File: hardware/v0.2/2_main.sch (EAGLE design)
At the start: 80 parts, among them IC1 SN74LVC1G08, IC2 FP6291, J1 RJ9PTH, Q1 PMOS, Q2 8050, Q3 MOSFET-NCHANNELBSS138, Q4 MOSFET-NCHANNELBSS138, U1 STM32F10XRXT6, Y1 8M

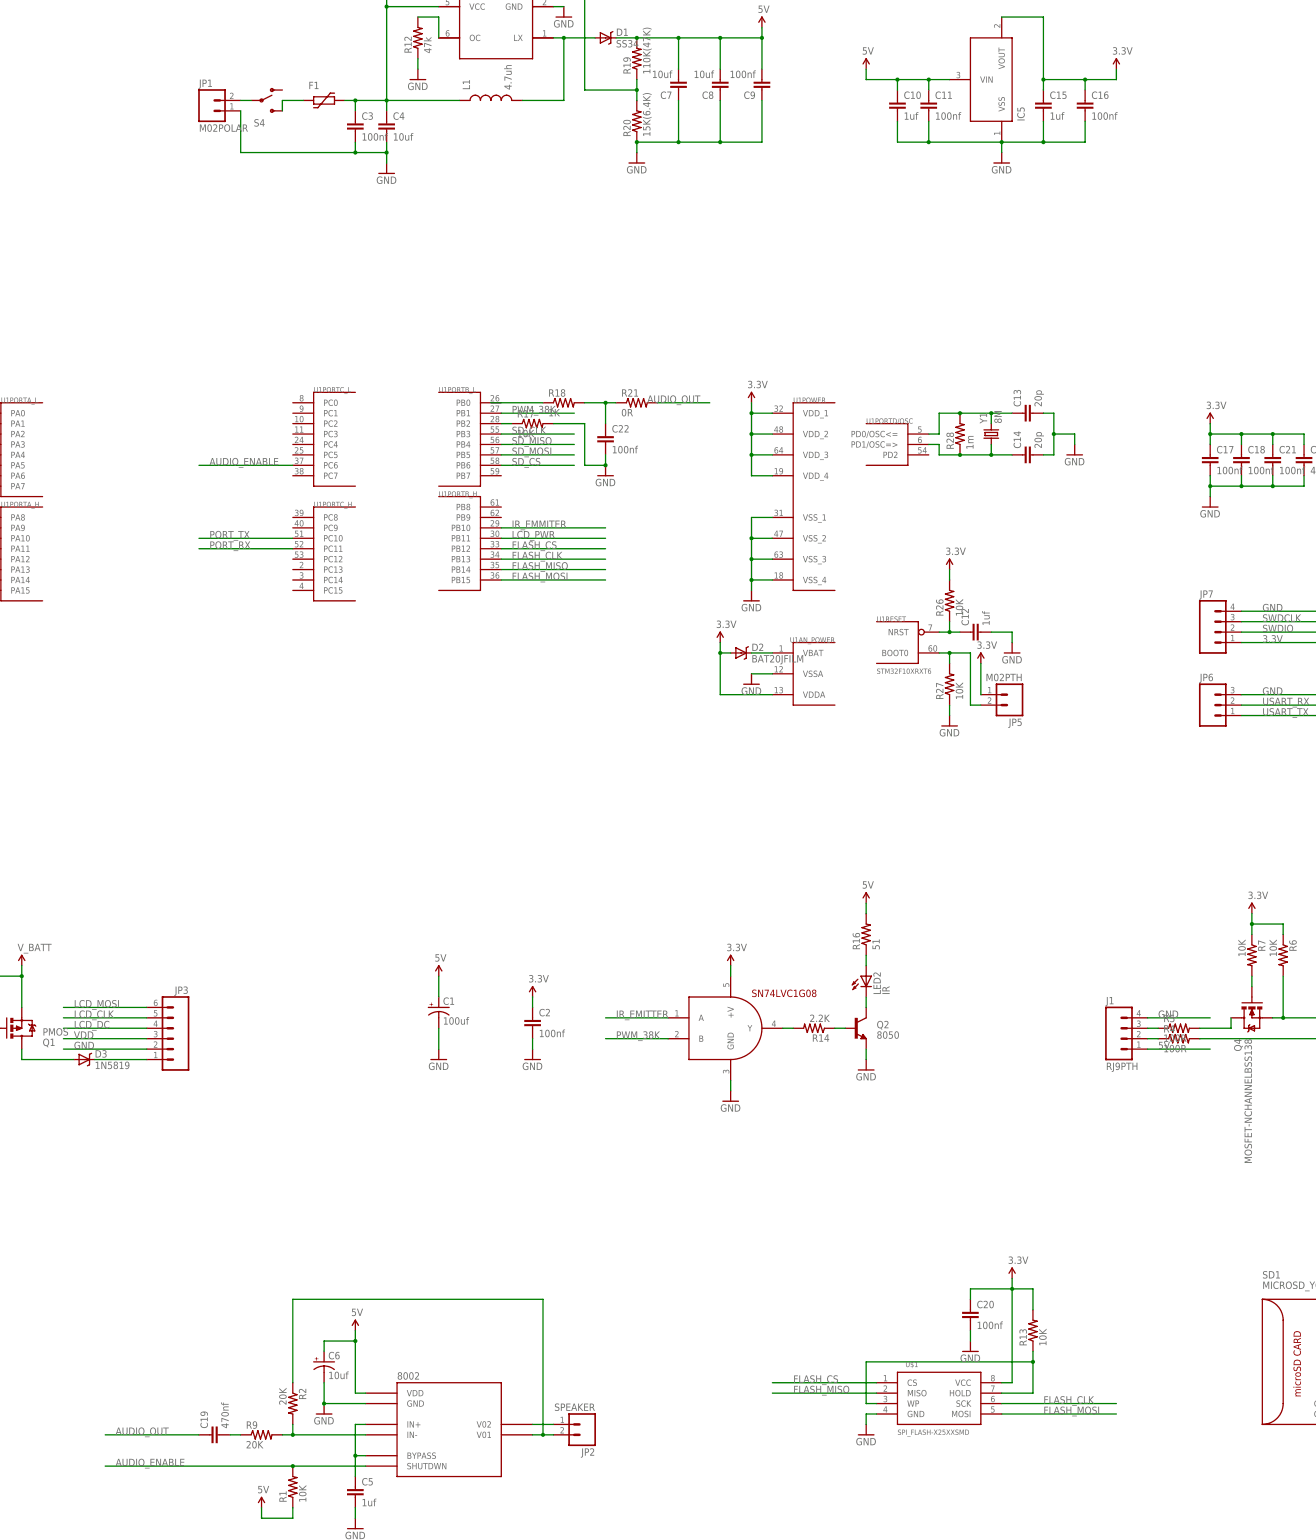
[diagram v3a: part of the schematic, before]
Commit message: update pcb
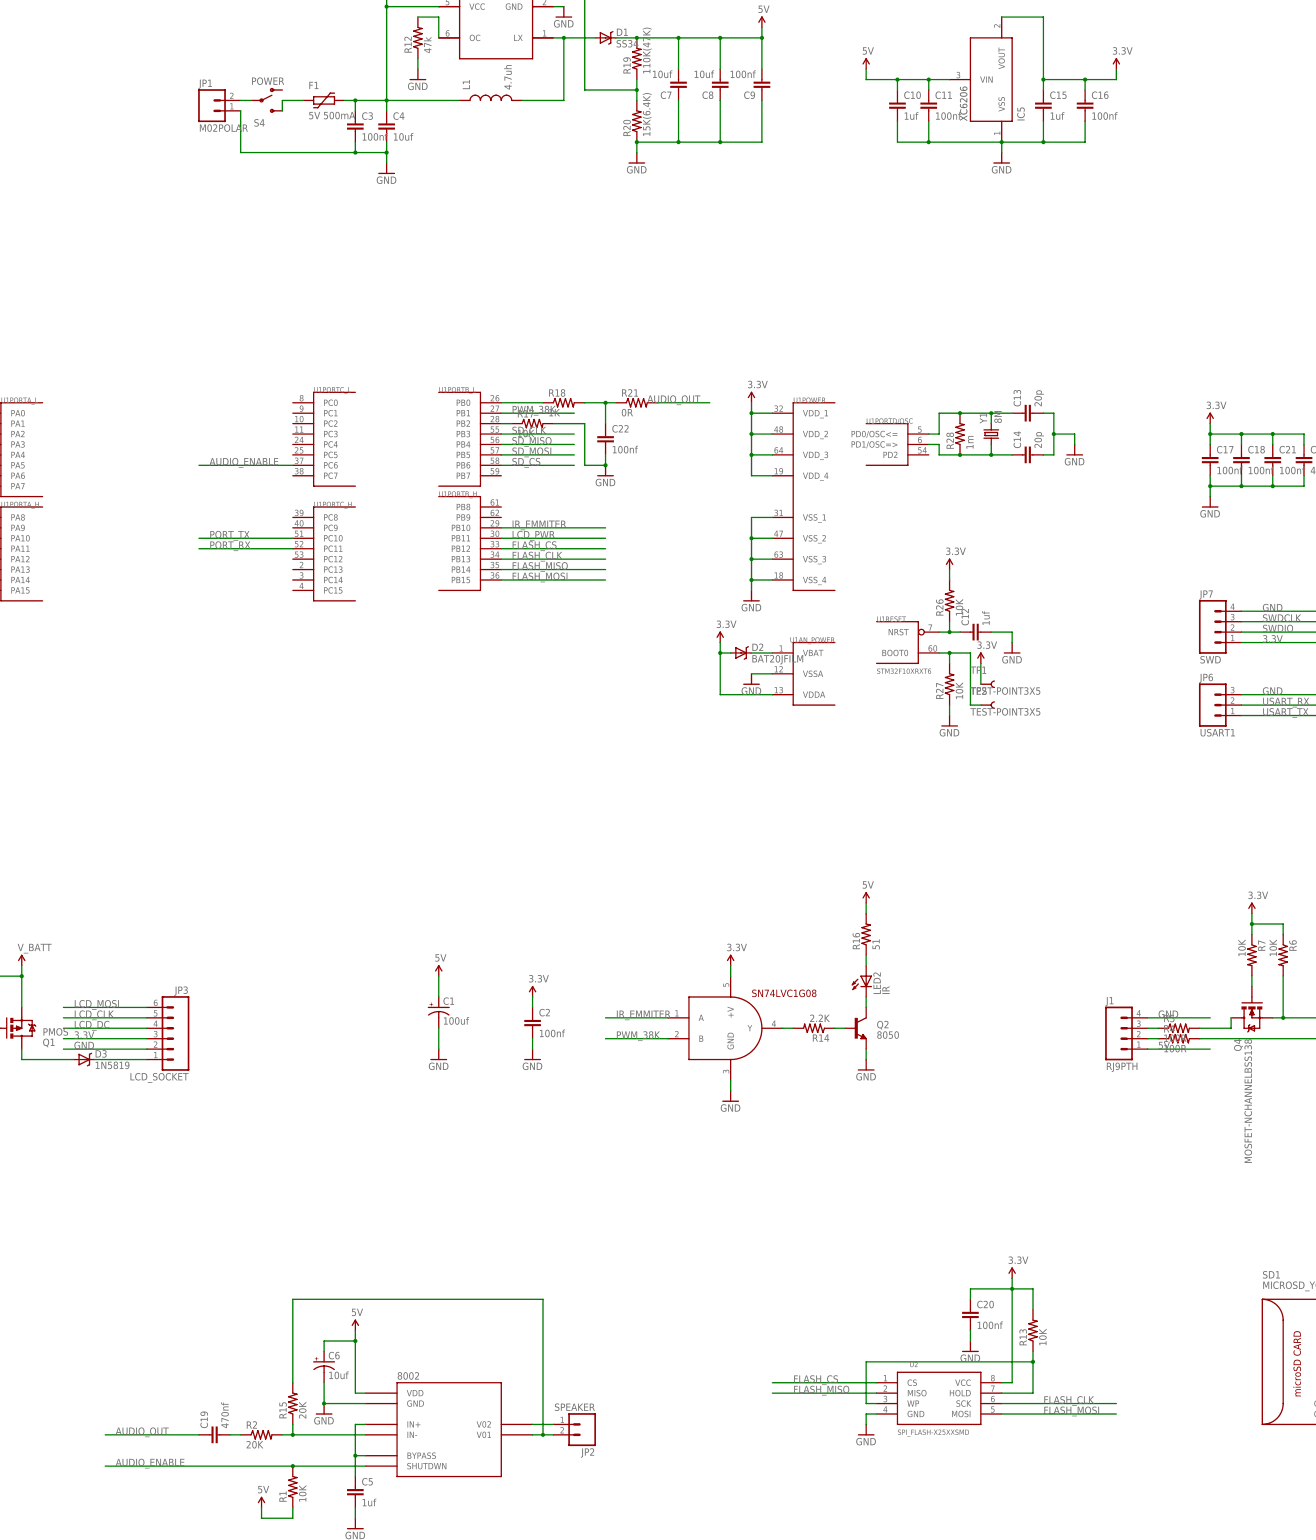
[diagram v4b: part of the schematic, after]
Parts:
- removed JP5: M02PTH, SparkFun-Connectors:M02PTH
- removed R9: 20K, SparkFun-Resistors:RESISTOR1206
- added R15: 20K, SparkFun-Passives:RESISTOR0603-RES
- added TP1, TP2: TEST-POINT3X5, SparkFun-Passives:TEST-POINT3X5
- F1: value (none) -> 5V 500mA
- IC5: value (none) -> XC6206
- JP3: value (none) -> LCD_SOCKET
- JP6: value (none) -> USART1
- JP7: value (none) -> SWD
- R1, R2: device SparkFun-Resistors:RESISTOR1206 -> SparkFun-Passives:RESISTOR0603-RES
- S4: value (none) -> POWER
- renumbered U$1 to U2
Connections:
- removed net IR_EMITTER: IC1.A
- removed net VDD: JP3.3
- net 3.3V: now also JP3.3, TP1.1; no longer JP5.1
- net AUDIO_ENABLE: now also U1PORTC_L.PC6
- net IR_EMMITER: now also IC1.A
- net N$14: now also U1PORTB_L.PB0
- net N$18: now also R15.2; no longer R2.1
- net N$19: now also R2.1; no longer R9.1
- net N$2: now also TP2.1; no longer JP5.2
- net N$21: now also R15.1; no longer R9.2
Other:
- moved on the sheet: R2
